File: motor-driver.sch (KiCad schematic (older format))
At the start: 19 parts, among them Q13 FDV304, SW1 SW_Push, SW3 SW_Push, SW4 SW_Push, U2 DRV8840

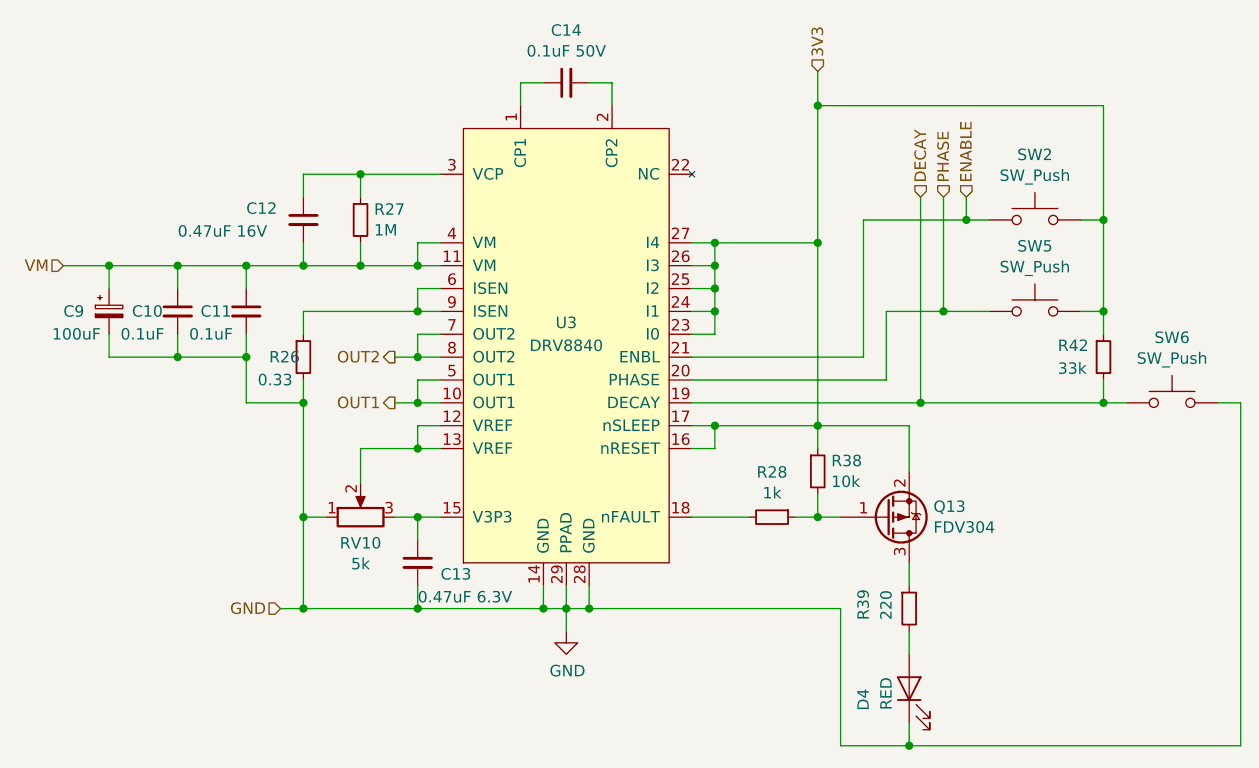
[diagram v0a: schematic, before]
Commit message: Routed all nets without GND. Added logo
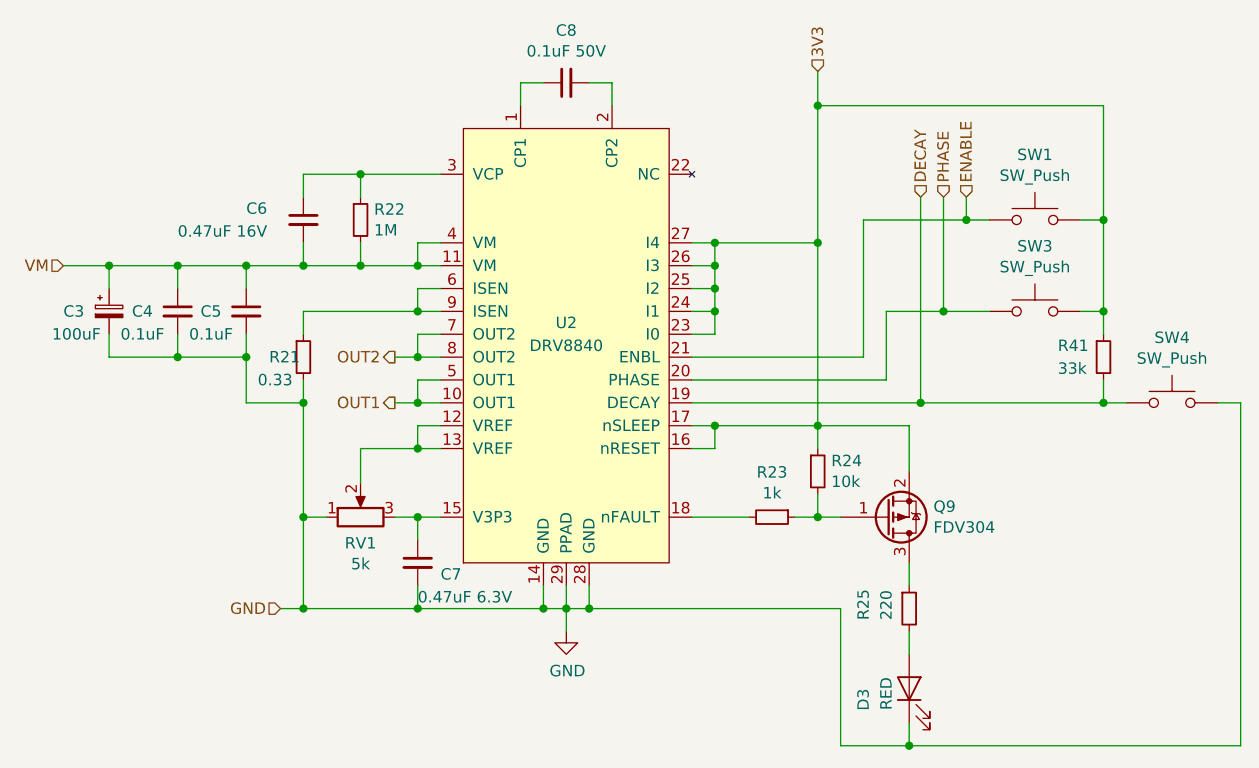
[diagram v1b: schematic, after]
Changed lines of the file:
@@
 $Descr A4 11693 8268
 encoding utf-8
-Sheet 7 8
+Sheet 5 8
 Title ""
 Date ""
@@
 AR Path="/5BDB64FF/5BE79BC7" Ref="R22"  Part="1"
 AR Path="/5C015BE4/5BE79BC7" Ref="R27"  Part="1"
-F 0 "R27" H 4509 3096 50  0000 L CNN
+F 0 "R22" H 4509 3096 50  0000 L CNN
 F 1 "1M" H 4509 3005 50  0000 L CNN
 F 2 "Resistor_SMD:R_0603_1608Metric" H 4450 3050 50  0001 C CNN
@@
 AR Path="/5BDB64FF/5BE79D59" Ref="C8"  Part="1"
 AR Path="/5C015BE4/5BE79D59" Ref="C14"  Part="1"
-F 0 "C14" V 5579 2450 50  0000 C CNN
+F 0 "C8" V 5579 2450 50  0000 C CNN
 F 1 "0.1uF 50V" V 5488 2450 50  0000 C CNN
 F 2 "Capacitor_SMD:C_0603_1608Metric" H 5350 2450 50  0001 C CNN
@@
 AR Path="/5BDB64FF/5BE7C590" Ref="C6"  Part="1"
 AR Path="/5C015BE4/5BE7C590" Ref="C12"  Part="1"
-F 0 "C12" H 3950 3100 50  0000 L CNN
+F 0 "C6" H 3950 3100 50  0000 L CNN
 F 1 "0.47uF 16V" H 3650 3000 50  0000 L CNN
 F 2 "Capacitor_SMD:C_0603_1608Metric" H 4200 3050 50  0001 C CNN
@@
 AR Path="/5BDB64FF/5BE78B4F" Ref="U2"  Part="1"
 AR Path="/5C015BE4/5BE78B4F" Ref="U3"  Part="1"
-F 0 "U3" H 5350 3700 50  0000 C CNN
+F 0 "U2" H 5350 3700 50  0000 C CNN
 F 1 "DRV8840" H 5350 3600 50  0000 C CNN
 F 2 "SOP65P640X110-29N:SOP65P640X110-29N" H 5200 3700 50  0001 C CNN
@@
 AR Path="/5BDB64FF/5BE7DEED" Ref="C5"  Part="1"
 AR Path="/5C015BE4/5BE7DEED" Ref="C11"  Part="1"
-F 0 "C11" H 3750 3450 50  0000 L CNN
+F 0 "C5" H 3750 3450 50  0000 L CNN
 F 1 "0.1uF" H 3700 3350 50  0000 L CNN
 F 2 "Capacitor_SMD:C_0603_1608Metric" H 3950 3450 50  0001 C CNN
@@
 AR Path="/5BDB64FF/5BE7DF37" Ref="C4"  Part="1"
 AR Path="/5C015BE4/5BE7DF37" Ref="C10"  Part="1"
-F 0 "C10" H 3450 3450 50  0000 L CNN
+F 0 "C4" H 3450 3450 50  0000 L CNN
 F 1 "0.1uF" H 3400 3350 50  0000 L CNN
 F 2 "Capacitor_SMD:C_0603_1608Metric" H 3650 3450 50  0001 C CNN
@@
 AR Path="/5BDB64FF/5BE7EFAF" Ref="C3"  Part="1"
 AR Path="/5C015BE4/5BE7EFAF" Ref="C9"  Part="1"
-F 0 "C9" H 3150 3450 50  0000 L CNN
+F 0 "C3" H 3150 3450 50  0000 L CNN
 F 1 "100uF" H 3100 3350 50  0000 L CNN
 F 2 "Capacitor_THT:CP_Radial_D6.3mm_P2.50mm" H 3350 3450 50  0001 C CNN
@@
 AR Path="/5BDB64FF/5BE7F85E" Ref="#PWR05"  Part="1"
 AR Path="/5C015BE4/5BE7F85E" Ref="#PWR07"  Part="1"
-F 0 "#PWR07" H 5350 4600 50  0001 C CNN
+F 0 "#PWR05" H 5350 4600 50  0001 C CNN
 F 1 "GND" H 5355 4677 50  0000 C CNN
 F 2 "" H 5350 4850 50  0001 C CNN
@@
 AR Path="/5BDB64FF/5BE84287" Ref="R21"  Part="1"
 AR Path="/5C015BE4/5BE84287" Ref="R26"  Part="1"
-F 0 "R26" H 4050 3650 50  0000 L CNN
+F 0 "R21" H 4050 3650 50  0000 L CNN
 F 1 "0.33" H 4000 3550 50  0000 L CNN
 F 2 "Resistor_SMD:R_2512_6332Metric" H 4200 3650 50  0001 C CNN
@@
 AR Path="/5BDB64FF/5BEAA7B3" Ref="R24"  Part="1"
 AR Path="/5C015BE4/5BEAA7B3" Ref="R38"  Part="1"
-F 0 "R38" H 6509 4196 50  0000 L CNN
+F 0 "R24" H 6509 4196 50  0000 L CNN
 F 1 "10k" H 6509 4105 50  0000 L CNN
 F 2 "Resistor_SMD:R_0603_1608Metric" H 6450 4150 50  0001 C CNN
@@
 AR Path="/5BDB64FF/5BEAD7B9" Ref="R23"  Part="1"
 AR Path="/5C015BE4/5BEAD7B9" Ref="R28"  Part="1"
-F 0 "R28" V 6054 4350 50  0000 C CNN
+F 0 "R23" V 6054 4350 50  0000 C CNN
 F 1 "1k" V 6145 4350 50  0000 C CNN
 F 2 "Resistor_SMD:R_0603_1608Metric" H 6250 4350 50  0001 C CNN
@@
 AR Path="/5BDB64FF/5BEB256D" Ref="D3"  Part="1"
 AR Path="/5C015BE4/5BEB256D" Ref="D4"  Part="1"
-F 0 "D4" H 6850 5300 50  0000 R CNN
+F 0 "D3" H 6850 5300 50  0000 R CNN
 F 1 "RED" H 6900 5200 50  0000 R CNN
 F 2 "LED_SMD:LED_0603_1608Metric_Castellated" H 6850 5100 50  0001 C CNN
@@
 AR Path="/5BDB64FF/5BEB7620" Ref="R25"  Part="1"
 AR Path="/5C015BE4/5BEB7620" Ref="R39"  Part="1"
-F 0 "R39" V 6650 4700 50  0000 L CNN
+F 0 "R25" V 6650 4700 50  0000 L CNN
 F 1 "220" V 6750 4700 50  0000 L CNN
 F 2 "Resistor_SMD:R_0603_1608Metric" H 6850 4750 50  0001 C CNN
@@
 AR Path="/5BDB64FF/5BECAFEA" Ref="C7"  Part="1"
 AR Path="/5C015BE4/5BECAFEA" Ref="C13"  Part="1"
-F 0 "C13" H 4800 4500 50  0000 L CNN
+F 0 "C7" H 4800 4500 50  0000 L CNN
 F 1 "0.47uF 6.3V" H 4700 4400 50  0000 L CNN
 F 2 "Capacitor_SMD:C_0603_1608Metric" H 4700 4550 50  0001 C CNN
@@
 AR Path="/5BDB64FF/5BE92513" Ref="RV1"  Part="1"
 AR Path="/5C015BE4/5BE92513" Ref="RV10"  Part="1"
-F 0 "RV10" V 4336 4350 50  0000 C CNN
+F 0 "RV1" V 4336 4350 50  0000 C CNN
 F 1 "5k" V 4245 4350 50  0000 C CNN
 F 2 "Potentiometer_THT:Potentiometer_Bourns_3266W_Vertical" H 4450 4350 50  0001 C CNN
@@
 AR Path="/5C015BE4/5BF252CB" Ref="Q13"  Part="1"
 AR Path="/5BDB64FF/5BF252CB" Ref="Q9"  Part="1"
-F 0 "Q13" H 6956 4304 50  0000 L CNN
+F 0 "Q9" H 6956 4304 50  0000 L CNN
 F 1 "FDV304" H 6956 4395 50  0000 L CNN
 F 2 "Package_TO_SOT_SMD:SOT-23" H 6950 4450 50  0001 C CNN
@@
 AR Path="/5BDB64FF/5BE949DE" Ref="SW1"  Part="1"
 AR Path="/5C015BE4/5BE949DE" Ref="SW2"  Part="1"
-F 0 "SW2" H 7400 3335 50  0000 C CNN
+F 0 "SW1" H 7400 3335 50  0000 C CNN
 F 1 "SW_Push" H 7400 3244 50  0000 C CNN
 F 2 "Button_Switch_SMD:SW_SPST_KMR2" H 7400 3250 50  0001 C CNN
@@
 AR Path="/5BDB64FF/5BE950B7" Ref="SW3"  Part="1"
 AR Path="/5C015BE4/5BE950B7" Ref="SW5"  Part="1"
-F 0 "SW5" H 7400 3735 50  0000 C CNN
+F 0 "SW3" H 7400 3735 50  0000 C CNN
 F 1 "SW_Push" H 7400 3644 50  0000 C CNN
 F 2 "Button_Switch_SMD:SW_SPST_KMR2" H 7400 3650 50  0001 C CNN
@@
 AR Path="/5BDB64FF/5BE950FD" Ref="SW4"  Part="1"
 AR Path="/5C015BE4/5BE950FD" Ref="SW6"  Part="1"
-F 0 "SW6" H 8000 4135 50  0000 C CNN
+F 0 "SW4" H 8000 4135 50  0000 C CNN
 F 1 "SW_Push" H 8000 4044 50  0000 C CNN
 F 2 "Button_Switch_SMD:SW_SPST_KMR2" H 8000 4050 50  0001 C CNN
@@
 AR Path="/5BDB64FF/5BEB4B1E" Ref="R41"  Part="1"
 AR Path="/5C015BE4/5BEB4B1E" Ref="R42"  Part="1"
-F 0 "R42" H 7500 3700 50  0000 L CNN
+F 0 "R41" H 7500 3700 50  0000 L CNN
 F 1 "33k" H 7500 3600 50  0000 L CNN
 F 2 "Resistor_SMD:R_0603_1608Metric" H 7700 3650 50  0001 C CNN

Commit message: Added switch for selecting Low/High power motor. Added thermal pads around motor controllers.
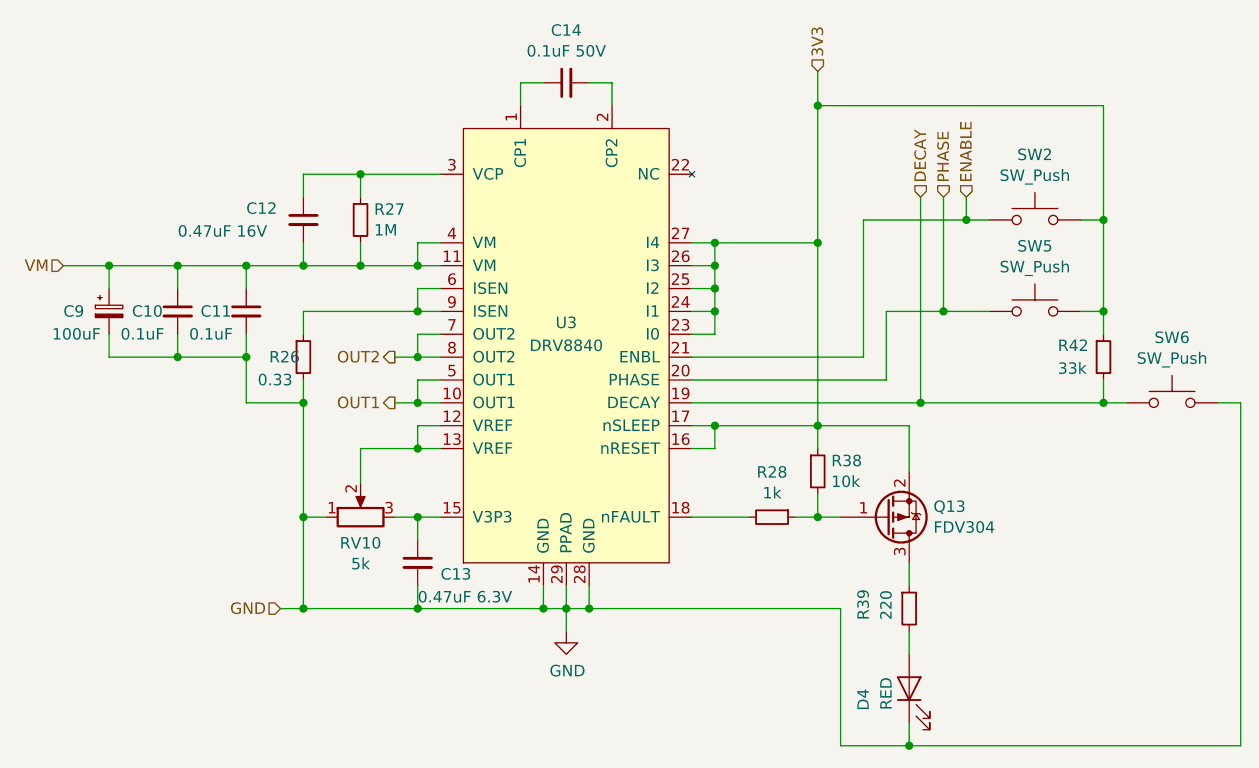
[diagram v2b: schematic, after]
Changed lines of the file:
@@
 $Descr A4 11693 8268
 encoding utf-8
-Sheet 5 8
+Sheet 7 8
 Title ""
 Date ""
@@
 AR Path="/5BDB64FF/5BE79BC7" Ref="R22"  Part="1"
 AR Path="/5C015BE4/5BE79BC7" Ref="R27"  Part="1"
-F 0 "R22" H 4509 3096 50  0000 L CNN
+F 0 "R27" H 4509 3096 50  0000 L CNN
 F 1 "1M" H 4509 3005 50  0000 L CNN
 F 2 "Resistor_SMD:R_0603_1608Metric" H 4450 3050 50  0001 C CNN
@@
 AR Path="/5BDB64FF/5BE79D59" Ref="C8"  Part="1"
 AR Path="/5C015BE4/5BE79D59" Ref="C14"  Part="1"
-F 0 "C8" V 5579 2450 50  0000 C CNN
+F 0 "C14" V 5579 2450 50  0000 C CNN
 F 1 "0.1uF 50V" V 5488 2450 50  0000 C CNN
 F 2 "Capacitor_SMD:C_0603_1608Metric" H 5350 2450 50  0001 C CNN
@@
 AR Path="/5BDB64FF/5BE7C590" Ref="C6"  Part="1"
 AR Path="/5C015BE4/5BE7C590" Ref="C12"  Part="1"
-F 0 "C6" H 3950 3100 50  0000 L CNN
+F 0 "C12" H 3950 3100 50  0000 L CNN
 F 1 "0.47uF 16V" H 3650 3000 50  0000 L CNN
 F 2 "Capacitor_SMD:C_0603_1608Metric" H 4200 3050 50  0001 C CNN
@@
 AR Path="/5BDB64FF/5BE78B4F" Ref="U2"  Part="1"
 AR Path="/5C015BE4/5BE78B4F" Ref="U3"  Part="1"
-F 0 "U2" H 5350 3700 50  0000 C CNN
+F 0 "U3" H 5350 3700 50  0000 C CNN
 F 1 "DRV8840" H 5350 3600 50  0000 C CNN
 F 2 "SOP65P640X110-29N:SOP65P640X110-29N" H 5200 3700 50  0001 C CNN
@@
 AR Path="/5BDB64FF/5BE7DEED" Ref="C5"  Part="1"
 AR Path="/5C015BE4/5BE7DEED" Ref="C11"  Part="1"
-F 0 "C5" H 3750 3450 50  0000 L CNN
+F 0 "C11" H 3750 3450 50  0000 L CNN
 F 1 "0.1uF" H 3700 3350 50  0000 L CNN
 F 2 "Capacitor_SMD:C_0603_1608Metric" H 3950 3450 50  0001 C CNN
@@
 AR Path="/5BDB64FF/5BE7DF37" Ref="C4"  Part="1"
 AR Path="/5C015BE4/5BE7DF37" Ref="C10"  Part="1"
-F 0 "C4" H 3450 3450 50  0000 L CNN
+F 0 "C10" H 3450 3450 50  0000 L CNN
 F 1 "0.1uF" H 3400 3350 50  0000 L CNN
 F 2 "Capacitor_SMD:C_0603_1608Metric" H 3650 3450 50  0001 C CNN
@@
 AR Path="/5BDB64FF/5BE7EFAF" Ref="C3"  Part="1"
 AR Path="/5C015BE4/5BE7EFAF" Ref="C9"  Part="1"
-F 0 "C3" H 3150 3450 50  0000 L CNN
+F 0 "C9" H 3150 3450 50  0000 L CNN
 F 1 "100uF" H 3100 3350 50  0000 L CNN
 F 2 "Capacitor_THT:CP_Radial_D6.3mm_P2.50mm" H 3350 3450 50  0001 C CNN
@@
 AR Path="/5BDB64FF/5BE7F85E" Ref="#PWR05"  Part="1"
 AR Path="/5C015BE4/5BE7F85E" Ref="#PWR07"  Part="1"
-F 0 "#PWR05" H 5350 4600 50  0001 C CNN
+F 0 "#PWR07" H 5350 4600 50  0001 C CNN
 F 1 "GND" H 5355 4677 50  0000 C CNN
 F 2 "" H 5350 4850 50  0001 C CNN
@@
 AR Path="/5BDB64FF/5BE84287" Ref="R21"  Part="1"
 AR Path="/5C015BE4/5BE84287" Ref="R26"  Part="1"
-F 0 "R21" H 4050 3650 50  0000 L CNN
+F 0 "R26" H 4050 3650 50  0000 L CNN
 F 1 "0.33" H 4000 3550 50  0000 L CNN
 F 2 "Resistor_SMD:R_2512_6332Metric" H 4200 3650 50  0001 C CNN
@@
 AR Path="/5BDB64FF/5BEAA7B3" Ref="R24"  Part="1"
 AR Path="/5C015BE4/5BEAA7B3" Ref="R38"  Part="1"
-F 0 "R24" H 6509 4196 50  0000 L CNN
+F 0 "R38" H 6509 4196 50  0000 L CNN
 F 1 "10k" H 6509 4105 50  0000 L CNN
 F 2 "Resistor_SMD:R_0603_1608Metric" H 6450 4150 50  0001 C CNN
@@
 AR Path="/5BDB64FF/5BEAD7B9" Ref="R23"  Part="1"
 AR Path="/5C015BE4/5BEAD7B9" Ref="R28"  Part="1"
-F 0 "R23" V 6054 4350 50  0000 C CNN
+F 0 "R28" V 6054 4350 50  0000 C CNN
 F 1 "1k" V 6145 4350 50  0000 C CNN
 F 2 "Resistor_SMD:R_0603_1608Metric" H 6250 4350 50  0001 C CNN
@@
 AR Path="/5BDB64FF/5BEB256D" Ref="D3"  Part="1"
 AR Path="/5C015BE4/5BEB256D" Ref="D4"  Part="1"
-F 0 "D3" H 6850 5300 50  0000 R CNN
+F 0 "D4" H 6850 5300 50  0000 R CNN
 F 1 "RED" H 6900 5200 50  0000 R CNN
 F 2 "LED_SMD:LED_0603_1608Metric_Castellated" H 6850 5100 50  0001 C CNN
@@
 AR Path="/5BDB64FF/5BEB7620" Ref="R25"  Part="1"
 AR Path="/5C015BE4/5BEB7620" Ref="R39"  Part="1"
-F 0 "R25" V 6650 4700 50  0000 L CNN
+F 0 "R39" V 6650 4700 50  0000 L CNN
 F 1 "220" V 6750 4700 50  0000 L CNN
 F 2 "Resistor_SMD:R_0603_1608Metric" H 6850 4750 50  0001 C CNN
@@
 AR Path="/5BDB64FF/5BECAFEA" Ref="C7"  Part="1"
 AR Path="/5C015BE4/5BECAFEA" Ref="C13"  Part="1"
-F 0 "C7" H 4800 4500 50  0000 L CNN
+F 0 "C13" H 4800 4500 50  0000 L CNN
 F 1 "0.47uF 6.3V" H 4700 4400 50  0000 L CNN
 F 2 "Capacitor_SMD:C_0603_1608Metric" H 4700 4550 50  0001 C CNN
@@
 AR Path="/5BDB64FF/5BE92513" Ref="RV1"  Part="1"
 AR Path="/5C015BE4/5BE92513" Ref="RV10"  Part="1"
-F 0 "RV1" V 4336 4350 50  0000 C CNN
+F 0 "RV10" V 4336 4350 50  0000 C CNN
 F 1 "5k" V 4245 4350 50  0000 C CNN
 F 2 "Potentiometer_THT:Potentiometer_Bourns_3266W_Vertical" H 4450 4350 50  0001 C CNN
@@
 AR Path="/5C015BE4/5BF252CB" Ref="Q13"  Part="1"
 AR Path="/5BDB64FF/5BF252CB" Ref="Q9"  Part="1"
-F 0 "Q9" H 6956 4304 50  0000 L CNN
+F 0 "Q13" H 6956 4304 50  0000 L CNN
 F 1 "FDV304" H 6956 4395 50  0000 L CNN
 F 2 "Package_TO_SOT_SMD:SOT-23" H 6950 4450 50  0001 C CNN
@@
 AR Path="/5BDB64FF/5BE949DE" Ref="SW1"  Part="1"
 AR Path="/5C015BE4/5BE949DE" Ref="SW2"  Part="1"
-F 0 "SW1" H 7400 3335 50  0000 C CNN
+F 0 "SW2" H 7400 3335 50  0000 C CNN
 F 1 "SW_Push" H 7400 3244 50  0000 C CNN
 F 2 "Button_Switch_SMD:SW_SPST_KMR2" H 7400 3250 50  0001 C CNN
@@
 AR Path="/5BDB64FF/5BE950B7" Ref="SW3"  Part="1"
 AR Path="/5C015BE4/5BE950B7" Ref="SW5"  Part="1"
-F 0 "SW3" H 7400 3735 50  0000 C CNN
+F 0 "SW5" H 7400 3735 50  0000 C CNN
 F 1 "SW_Push" H 7400 3644 50  0000 C CNN
 F 2 "Button_Switch_SMD:SW_SPST_KMR2" H 7400 3650 50  0001 C CNN
@@
 AR Path="/5BDB64FF/5BE950FD" Ref="SW4"  Part="1"
 AR Path="/5C015BE4/5BE950FD" Ref="SW6"  Part="1"
-F 0 "SW4" H 8000 4135 50  0000 C CNN
+F 0 "SW6" H 8000 4135 50  0000 C CNN
 F 1 "SW_Push" H 8000 4044 50  0000 C CNN
 F 2 "Button_Switch_SMD:SW_SPST_KMR2" H 8000 4050 50  0001 C CNN
@@
 AR Path="/5BDB64FF/5BEB4B1E" Ref="R41"  Part="1"
 AR Path="/5C015BE4/5BEB4B1E" Ref="R42"  Part="1"
-F 0 "R41" H 7500 3700 50  0000 L CNN
+F 0 "R42" H 7500 3700 50  0000 L CNN
 F 1 "33k" H 7500 3600 50  0000 L CNN
 F 2 "Resistor_SMD:R_0603_1608Metric" H 7700 3650 50  0001 C CNN
